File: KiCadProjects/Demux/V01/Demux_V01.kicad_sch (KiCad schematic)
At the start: 40 parts, among them J1 alimentacao analogica, J12 +9Vmux, J13 +5Vmux, J14 +3.3Vmux, J15 -9Vmux, J16 -5Vmux, J17 GNDmux, J18 Conn_01x03, J19 Conn_01x06, J2 sinais analogicos, J20 Conn_01x06, J21 Conn_01x06, J22 Conn_01x06, J23 Conn_01x06, J24 Conn_01x06, J25 Conn_01x06, J26 Conn_01x06, J27 Conn_01x06, J28 Conn_01x06, J29 Conn_01x06, J3 comunicacao / sinais digitais, J30 Conn_01x06, J31 Conn_01x06, J32 Conn_01x06, J33 Conn_01x06, J34 Conn_01x06, J4 Conn_01x02, J5 Conn_01x02, J6 Conn_01x02, U1A1 74HC4051, U1B1 74HC4051, U2 BluePill_STM32F103C, U2A2 74HC4051, U2B2 74HC4051, U3A3 74HC4051, U3B3 74HC4051, U4A4 74HC4051, U4B4 74HC4051, U5A1 74HC4051, U5B1 74HC4051

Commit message: modificar
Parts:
- J12, J13, J14, J15, J16, J17, J4, J5, J6: footprint (none) -> Connector_PinHeader_2.54mm:PinHeader_1x02_P2.54mm_Vertical
- J18: footprint (none) -> Connector_PinHeader_2.54mm:PinHeader_1x03_P2.54mm_Vertical
- J19, J20, J21, J22, J23, J24, J25, J26, J27, J28, J29, J30, J31, J32, J33, J34: footprint (none) -> Connector_PinHeader_2.54mm:PinHeader_1x06_P2.54mm_Horizontal
- U1A1, U1B1, U2A2, U2B2, U3A3, U3B3, U4A4, U4B4, U5A1, U5B1: footprint (none) -> 74HC4051N:N16
- U2: footprint BluePill_breakouts:BluePill_STM32F103C -> BluePill_STM32:BluePill_STM32F103C
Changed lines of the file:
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@@
       (effects (font (size 1.27 1.27)))
     )
-    (property "Footprint" "" (at 224.663 51.181 0)
+    (property "Footprint" "Connector_PinHeader_2.54mm:PinHeader_1x06_P2.54mm_Horizontal" (at 224.663 51.181 0)
       (effects (font (size 1.27 1.27)) hide)
     )
@@
       (effects (font (size 1.27 1.27)) (justify left))
     )
-    (property "Footprint" "" (at 26.924 60.706 0)
+    (property "Footprint" "74HC4051N:N16" (at 26.924 60.706 0)
       (effects (font (size 1.27 1.27)) hide)
     )
@@
       (effects (font (size 1.27 1.27)))
     )
-    (property "Footprint" "" (at 257.302 25.781 0)
+    (property "Footprint" "Connector_PinHeader_2.54mm:PinHeader_1x06_P2.54mm_Horizontal" (at 257.302 25.781 0)
       (effects (font (size 1.27 1.27)) hide)
     )
@@
       (effects (font (size 1.27 1.27)))
     )
-    (property "Footprint" "" (at 144.272 122.428 0)
+    (property "Footprint" "Connector_PinHeader_2.54mm:PinHeader_1x02_P2.54mm_Vertical" (at 144.272 122.428 0)
       (effects (font (size 1.27 1.27)) hide)
     )
@@
       (effects (font (size 1.27 1.27)))
     )
-    (property "Footprint" "" (at 224.663 25.654 0)
+    (property "Footprint" "Connector_PinHeader_2.54mm:PinHeader_1x06_P2.54mm_Horizontal" (at 224.663 25.654 0)
       (effects (font (size 1.27 1.27)) hide)
     )
@@
       (effects (font (size 1.27 1.27)) (justify left))
     )
-    (property "Footprint" "" (at 27.432 134.874 0)
+    (property "Footprint" "74HC4051N:N16" (at 27.432 134.874 0)
       (effects (font (size 1.27 1.27)) hide)
     )
@@
       (effects (font (size 1.27 1.27)))
     )
-    (property "Footprint" "" (at 273.685 25.781 0)
+    (property "Footprint" "Connector_PinHeader_2.54mm:PinHeader_1x06_P2.54mm_Horizontal" (at 273.685 25.781 0)
       (effects (font (size 1.27 1.27)) hide)
     )
@@
       (effects (font (size 1.27 1.27)))
     )
-    (property "Footprint" "" (at 273.685 51.308 0)
+    (property "Footprint" "Connector_PinHeader_2.54mm:PinHeader_1x06_P2.54mm_Horizontal" (at 273.685 51.308 0)
       (effects (font (size 1.27 1.27)) hide)
     )
@@
       (effects (font (size 1.27 1.27)) (justify left))
     )
-    (property "Footprint" "" (at 107.95 77.724 0)
+    (property "Footprint" "74HC4051N:N16" (at 107.95 77.724 0)
       (effects (font (size 1.27 1.27)) hide)
     )
@@
       (effects (font (size 1.27 1.27)) (justify left))
     )
-    (property "Footprint" "" (at 103.378 156.972 0)
+    (property "Footprint" "74HC4051N:N16" (at 103.378 156.972 0)
       (effects (font (size 1.27 1.27)) hide)
     )
@@
       (effects (font (size 1.27 1.27)))
     )
-    (property "Footprint" "" (at 179.324 125.984 0)
+    (property "Footprint" "Connector_PinHeader_2.54mm:PinHeader_1x02_P2.54mm_Vertical" (at 179.324 125.984 0)
       (effects (font (size 1.27 1.27)) hide)
     )
@@
       (effects (font (size 1.27 1.27)))
     )
-    (property "Footprint" "" (at 224.409 75.5142 0)
+    (property "Footprint" "Connector_PinHeader_2.54mm:PinHeader_1x06_P2.54mm_Horizontal" (at 224.409 75.5142 0)
       (effects (font (size 1.27 1.27)) hide)
     )
@@
       (effects (font (size 1.27 1.27)))
     )
-    (property "Footprint" "BluePill_breakouts:BluePill_STM32F103C" (at 164.592 16.256 0)
+    (property "Footprint" "BluePill_STM32:BluePill_STM32F103C" (at 164.592 16.256 0)
       (effects (font (size 1.27 1.27)) hide)
     )
@@
       (effects (font (size 1.27 1.27)) (justify left))
     )
-    (property "Footprint" "" (at 65.786 74.168 0)
+    (property "Footprint" "74HC4051N:N16" (at 65.786 74.168 0)
       (effects (font (size 1.27 1.27)) hide)
     )
@@
       (effects (font (size 1.27 1.27)))
     )
-    (property "Footprint" "" (at 160.528 147.574 0)
+    (property "Footprint" "Connector_PinHeader_2.54mm:PinHeader_1x02_P2.54mm_Vertical" (at 160.528 147.574 0)
       (effects (font (size 1.27 1.27)) hide)
     )
@@
       (effects (font (size 1.27 1.27)) (justify left))
     )
-    (property "Footprint" "" (at 106.426 41.656 0)
+    (property "Footprint" "74HC4051N:N16" (at 106.426 41.656 0)
       (effects (font (size 1.27 1.27)) hide)
     )
@@
       (effects (font (size 1.27 1.27)))
     )
-    (property "Footprint" "" (at 150.114 147.574 0)
+    (property "Footprint" "Connector_PinHeader_2.54mm:PinHeader_1x02_P2.54mm_Vertical" (at 150.114 147.574 0)
       (effects (font (size 1.27 1.27)) hide)
     )
@@
       (effects (font (size 1.27 1.27)) (justify left))
     )
-    (property "Footprint" "" (at 63.246 113.792 0)
+    (property "Footprint" "74HC4051N:N16" (at 63.246 113.792 0)
       (effects (font (size 1.27 1.27)) hide)
     )
@@
       (effects (font (size 1.27 1.27)))
     )
-    (property "Footprint" "" (at 155.956 122.682 0)
+    (property "Footprint" "Connector_PinHeader_2.54mm:PinHeader_1x02_P2.54mm_Vertical" (at 155.956 122.682 0)
       (effects (font (size 1.27 1.27)) hide)
     )
@@
       (effects (font (size 1.27 1.27)))
     )
-    (property "Footprint" "" (at 257.048 75.6412 0)
+    (property "Footprint" "Connector_PinHeader_2.54mm:PinHeader_1x06_P2.54mm_Horizontal" (at 257.048 75.6412 0)
       (effects (font (size 1.27 1.27)) hide)
     )
@@
       (effects (font (size 1.27 1.27)))
     )
-    (property "Footprint" "" (at 240.919 25.654 0)
+    (property "Footprint" "Connector_PinHeader_2.54mm:PinHeader_1x06_P2.54mm_Horizontal" (at 240.919 25.654 0)
       (effects (font (size 1.27 1.27)) hide)
     )
@@
       (effects (font (size 1.27 1.27)))
     )
-    (property "Footprint" "" (at 131.318 122.682 0)
+    (property "Footprint" "Connector_PinHeader_2.54mm:PinHeader_1x02_P2.54mm_Vertical" (at 131.318 122.682 0)
       (effects (font (size 1.27 1.27)) hide)
     )
@@
       (effects (font (size 1.27 1.27)) (justify left))
     )
-    (property "Footprint" "" (at 62.23 153.162 0)
+    (property "Footprint" "74HC4051N:N16" (at 62.23 153.162 0)
       (effects (font (size 1.27 1.27)) hide)
     )
@@
       (effects (font (size 1.27 1.27)))
     )
-    (property "Footprint" "" (at 171.704 148.082 0)
+    (property "Footprint" "Connector_PinHeader_2.54mm:PinHeader_1x02_P2.54mm_Vertical" (at 171.704 148.082 0)
       (effects (font (size 1.27 1.27)) hide)
     )
@@
       (effects (font (size 1.27 1.27)))
     )
-    (property "Footprint" "" (at 240.919 51.181 0)
+    (property "Footprint" "Connector_PinHeader_2.54mm:PinHeader_1x06_P2.54mm_Horizontal" (at 240.919 51.181 0)
       (effects (font (size 1.27 1.27)) hide)
     )
@@
       (effects (font (size 1.27 1.27)))
     )
-    (property "Footprint" "" (at 224.536 97.79 0)
+    (property "Footprint" "Connector_PinHeader_2.54mm:PinHeader_1x06_P2.54mm_Horizontal" (at 224.536 97.79 0)
       (effects (font (size 1.27 1.27)) hide)
     )
@@
       (effects (font (size 1.27 1.27)))
     )
-    (property "Footprint" "" (at 166.37 126.238 0)
+    (property "Footprint" "Connector_PinHeader_2.54mm:PinHeader_1x02_P2.54mm_Vertical" (at 166.37 126.238 0)
       (effects (font (size 1.27 1.27)) hide)
     )
@@
       (effects (font (size 1.27 1.27)))
     )
-    (property "Footprint" "" (at 273.812 98.044 0)
+    (property "Footprint" "Connector_PinHeader_2.54mm:PinHeader_1x06_P2.54mm_Horizontal" (at 273.812 98.044 0)
       (effects (font (size 1.27 1.27)) hide)
     )
@@
       (effects (font (size 1.27 1.27)) (justify left))
     )
-    (property "Footprint" "" (at 30.988 106.172 0)
+    (property "Footprint" "Connector_PinHeader_2.54mm:PinHeader_1x03_P2.54mm_Vertical" (at 30.988 106.172 0)
       (effects (font (size 1.27 1.27)) hide)
     )
@@
       (effects (font (size 1.27 1.27)))
     )
-    (property "Footprint" "" (at 240.3856 75.4888 0)
+    (property "Footprint" "Connector_PinHeader_2.54mm:PinHeader_1x06_P2.54mm_Horizontal" (at 240.3856 75.4888 0)
       (effects (font (size 1.27 1.27)) hide)
     )
@@
       (effects (font (size 1.27 1.27)))
     )
-    (property "Footprint" "" (at 273.05 75.692 0)
+    (property "Footprint" "Connector_PinHeader_2.54mm:PinHeader_1x06_P2.54mm_Horizontal" (at 273.05 75.692 0)
       (effects (font (size 1.27 1.27)) hide)
     )
@@
       (effects (font (size 1.27 1.27)))
     )
-    (property "Footprint" "" (at 257.302 51.308 0)
+    (property "Footprint" "Connector_PinHeader_2.54mm:PinHeader_1x06_P2.54mm_Horizontal" (at 257.302 51.308 0)
       (effects (font (size 1.27 1.27)) hide)
     )
@@
       (effects (font (size 1.27 1.27)))
     )
-    (property "Footprint" "" (at 257.302 97.79 0)
+    (property "Footprint" "Connector_PinHeader_2.54mm:PinHeader_1x06_P2.54mm_Horizontal" (at 257.302 97.79 0)
       (effects (font (size 1.27 1.27)) hide)
     )
@@
       (effects (font (size 1.27 1.27)) (justify left))
     )
-    (property "Footprint" "" (at 102.108 118.872 0)
+    (property "Footprint" "74HC4051N:N16" (at 102.108 118.872 0)
       (effects (font (size 1.27 1.27)) hide)
     )
@@
       (effects (font (size 1.27 1.27)))
     )
-    (property "Footprint" "" (at 240.792 97.79 0)
+    (property "Footprint" "Connector_PinHeader_2.54mm:PinHeader_1x06_P2.54mm_Horizontal" (at 240.792 97.79 0)
       (effects (font (size 1.27 1.27)) hide)
     )
@@
       (effects (font (size 1.27 1.27)) (justify left))
     )
-    (property "Footprint" "" (at 66.04 39.624 0)
+    (property "Footprint" "74HC4051N:N16" (at 66.04 39.624 0)
       (effects (font (size 1.27 1.27)) hide)
     )
@@
       (effects (font (size 1.27 1.27)))
     )
-    (property "Footprint" "" (at 191.008 126.238 0)
+    (property "Footprint" "Connector_PinHeader_2.54mm:PinHeader_1x02_P2.54mm_Vertical" (at 191.008 126.238 0)
       (effects (font (size 1.27 1.27)) hide)
     )

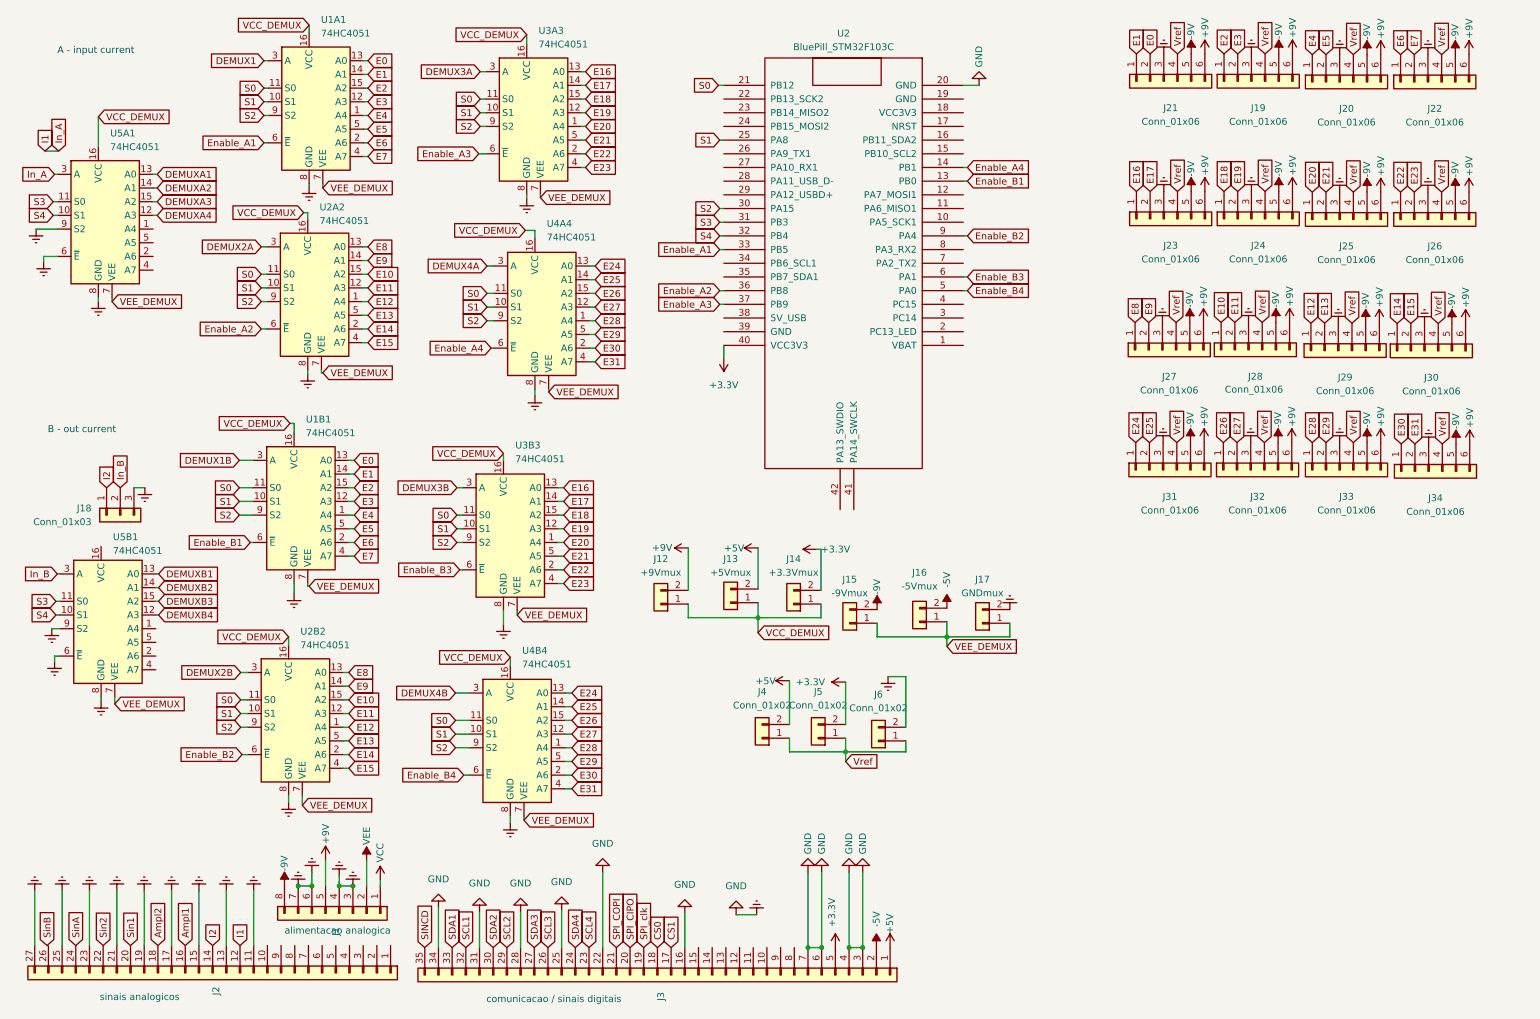
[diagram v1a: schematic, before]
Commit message: placa em producao
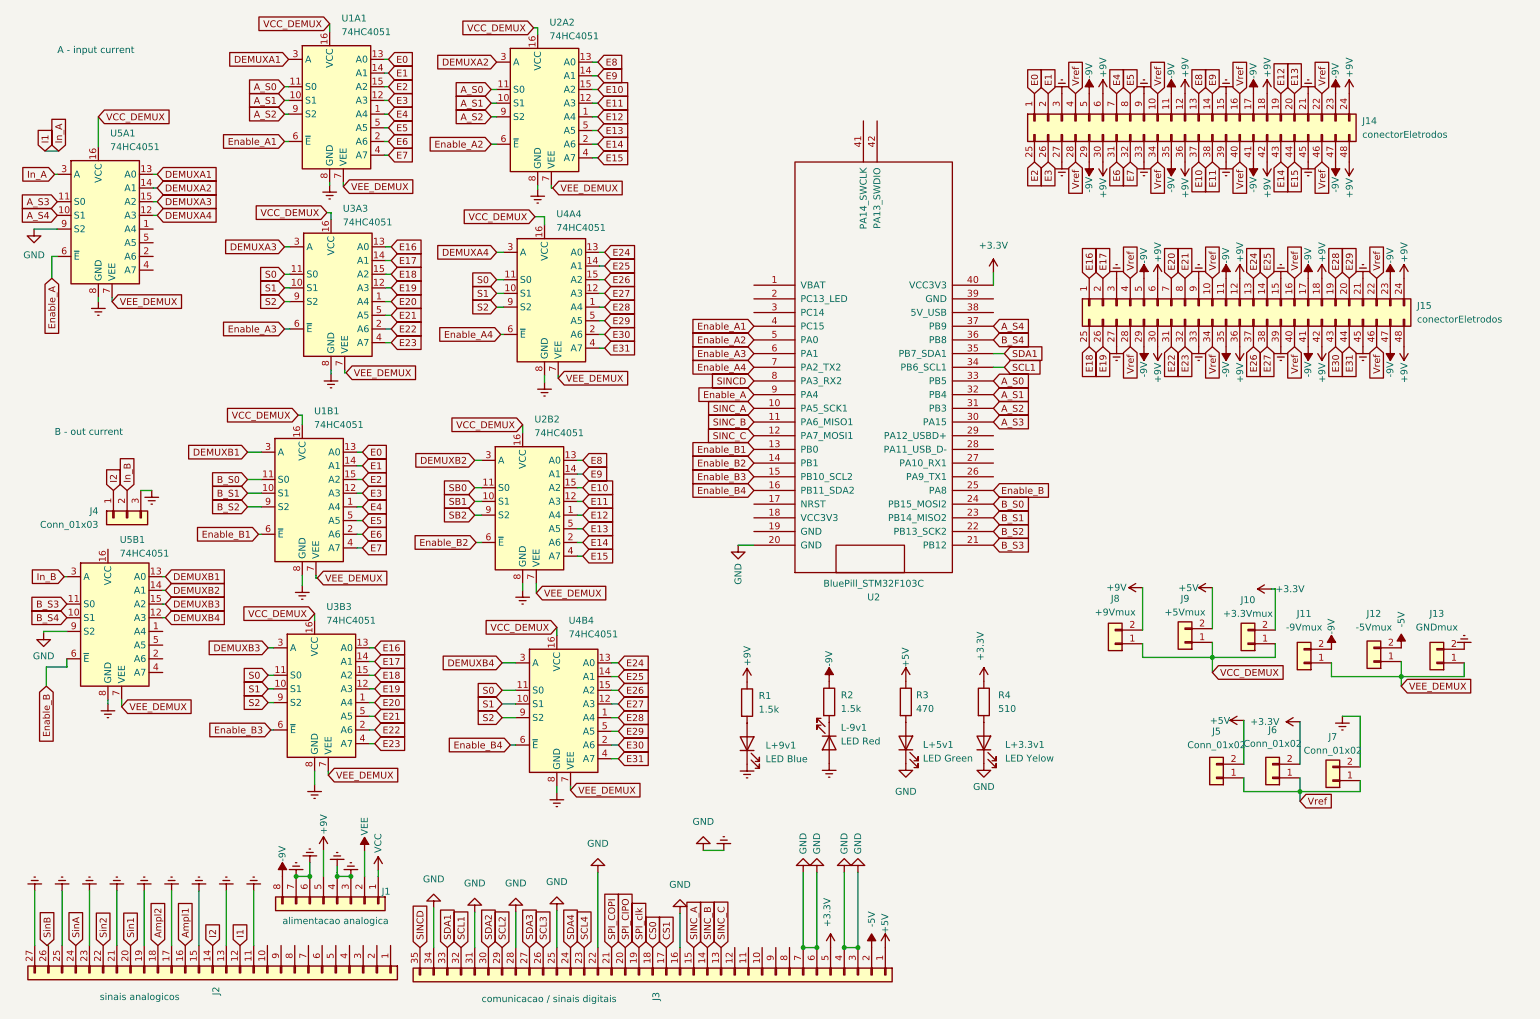
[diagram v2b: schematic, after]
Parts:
- removed J19, J20, J21, J22, J23, J24, J25, J26, J27, J28, J29, J30, J31, J32, J33, J34: Conn_01x06, Connector_PinHeader_2.54mm:PinHeader_1x06_P2.54mm_Horizontal, symbol Connector_Generic:Conn_01x06
- added J14, J15: conectorEletrodos, Connector_PinHeader_2.54mm:PinHeader_2x24_P2.54mm_Vertical, symbol Connector_Generic:Conn_02x24_Top_Bottom
- added L+3.3v1: LED Yelow, LED_THT:LED_D5.0mm, symbol Device:LED
- added L+5v1: LED Green, LED_THT:LED_D5.0mm, symbol Device:LED
- added L+9v1: LED Blue, LED_THT:LED_D5.0mm, symbol Device:LED
- added L-9v1: LED Red, LED_THT:LED_D5.0mm, symbol Device:LED
- added R1, R2: 1.5k, Resistor_THT:R_Axial_DIN0207_L6.3mm_D2.5mm_P7.62mm_Horizontal, symbol Device:R
- added R3: 470, Resistor_THT:R_Axial_DIN0207_L6.3mm_D2.5mm_P7.62mm_Horizontal, symbol Device:R
- added R4: 510, Resistor_THT:R_Axial_DIN0207_L6.3mm_D2.5mm_P7.62mm_Horizontal, symbol Device:R
- renumbered J14 to J10, J15 to J11, J16 to J12, J17 to J13, J18 to J4, J4 to J5, J5 to J6, J6 to J7, J12 to J8, J13 to J9
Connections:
- net DEMUX1 is gone; now on net DEMUXA1: U1A1.3 (A)
- net DEMUX1B is gone; now on net DEMUXB1: U1B1.3 (A)
- net DEMUX2A is gone; now on net DEMUXA2: U2A2.3 (A)
- net DEMUX2B is gone; now on net DEMUXB2: U2B2.3 (A)
- net DEMUX3A is gone; now on net DEMUXA3: U3A3.3 (A)
- net DEMUX3B is gone; now on net DEMUXB3: U3B3.3 (A)
- net DEMUX4A is gone; now on net DEMUXA4: U4A4.3 (A)
- net DEMUX4B is gone; now on net DEMUXB4: U4B4.3 (A)
- net +3.3V: now also R4.1
- net +5V: now also R3.1
- net +9V: now also J14.12 (Pin_12), J14.18 (Pin_18), J14.24 (Pin_24), J14.30 (Pin_30), J14.36 (Pin_36), J14.42 (Pin_42), J14.48 (Pin_48), J14.6 (Pin_6), J15.12 (Pin_12), J15.18 (Pin_18), J15.24 (Pin_24), J15.30 (Pin_30), J15.36 (Pin_36), J15.42 (Pin_42), J15.48 (Pin_48), J15.6 (Pin_6), R1.1
- net -9V: now also J14.11 (Pin_11), J14.17 (Pin_17), J14.23 (Pin_23), J14.29 (Pin_29), J14.35 (Pin_35), J14.41 (Pin_41), J14.47 (Pin_47), J14.5 (Pin_5), J15.11 (Pin_11), J15.17 (Pin_17), J15.23 (Pin_23), J15.29 (Pin_29), J15.35 (Pin_35), J15.41 (Pin_41), J15.47 (Pin_47), J15.5 (Pin_5), R2.1
- net E0: now also J14.1 (Pin_1)
- net E1: now also J14.2 (Pin_2)
- net E10: now also J14.37 (Pin_37)
- net E11: now also J14.38 (Pin_38)
- net E12: now also J14.19 (Pin_19)
- net E13: now also J14.20 (Pin_20)
- net E14: now also J14.43 (Pin_43)
- net E15: now also J14.44 (Pin_44)
- net E16: now also J15.1 (Pin_1)
- net E17: now also J15.2 (Pin_2)
- net E18: now also J15.25 (Pin_25)
- net E19: now also J15.26 (Pin_26)
- net E2: now also J14.25 (Pin_25)
- net E20: now also J15.7 (Pin_7)
- net E21: now also J15.8 (Pin_8)
- net E22: now also J15.31 (Pin_31)
- net E23: now also J15.32 (Pin_32)
- net E24: now also J15.13 (Pin_13)
- net E25: now also J15.14 (Pin_14)
- net E26: now also J15.37 (Pin_37)
- net E27: now also J15.38 (Pin_38)
- net E28: now also J15.19 (Pin_19)
- net E29: now also J15.20 (Pin_20)
- net E3: now also J14.26 (Pin_26)
- net E30: now also J15.43 (Pin_43)
- net E31: now also J15.44 (Pin_44)
- net E4: now also J14.7 (Pin_7)
- net E5: now also J14.8 (Pin_8)
- net E6: now also J14.31 (Pin_31)
- net E7: now also J14.32 (Pin_32)
- net E8: now also J14.13 (Pin_13)
- net E9: now also J14.14 (Pin_14)
- net Earth: now also J14.15 (Pin_15), J14.21 (Pin_21), J14.27 (Pin_27), J14.3 (Pin_3), J14.33 (Pin_33), J14.39 (Pin_39), J14.45 (Pin_45), J14.9 (Pin_9), J15.15 (Pin_15), J15.21 (Pin_21), J15.27 (Pin_27), J15.3 (Pin_3), J15.33 (Pin_33), J15.39 (Pin_39), J15.45 (Pin_45), J15.9 (Pin_9), L+3.3v1.1 (K), L+5v1.1 (K), L+9v1.1 (K), L-9v1.2 (A); no longer U5A1.6 (~{E}), U5B1.6 (~{E})
- net Enable_A1: now also U2.4 (PC15); no longer U2.33 (PB5)
- net Enable_A2: now also U2.5 (PA0); no longer U2.36 (PB8)
- net Enable_A3: now also U2.6 (PA1); no longer U2.37 (PB9)
- net Enable_A4: now also U2.7 (PA2_TX2); no longer U2.14 (PB1)
- net Enable_B2: now also U2.14 (PB1); no longer U2.9 (PA4)
- net Enable_B3: now also U2.15 (PB10_SCL2); no longer U2.6 (PA1)
- net Enable_B4: now also U2.16 (PB11_SDA2); no longer U2.5 (PA0)
- net S0: no longer U1A1.11 (S0), U1B1.11 (S0), U2.21 (PB12), U2A2.11 (S0), U2B2.11 (S0)
- net S1: no longer U1A1.10 (S1), U1B1.10 (S1), U2.25 (PA8), U2A2.10 (S1), U2B2.10 (S1)
- net S2: no longer U1A1.9 (S2), U1B1.9 (S2), U2.30 (PA15), U2A2.9 (S2), U2B2.9 (S2)
- net SCL1: now also U2.34 (PB6_SCL1)
- net SDA1: now also U2.35 (PB7_SDA1)
- net SINCD: now also U2.8 (PA3_RX2)
- net Vref: now also J14.10 (Pin_10), J14.16 (Pin_16), J14.22 (Pin_22), J14.28 (Pin_28), J14.34 (Pin_34), J14.4 (Pin_4), J14.40 (Pin_40), J14.46 (Pin_46), J15.10 (Pin_10), J15.16 (Pin_16), J15.22 (Pin_22), J15.28 (Pin_28), J15.34 (Pin_34), J15.4 (Pin_4), J15.40 (Pin_40), J15.46 (Pin_46)
- net SINC_A: now reaches U2.10 (PA5_SCK1)
- net SINC_A: now also J3.15 (Pin_15)
- net SINC_B: now reaches U2.11 (PA6_MISO1)
- net SINC_B: now also J3.14 (Pin_14)
- net SINC_C: now reaches U2.12 (PA7_MOSI1)
- net SINC_C: now also J3.13 (Pin_13)
- net B_S2: now reaches U2.22 (PB13_SCK2)
- net B_S2: now also U1B1.9 (S2)
- net B_S1: now reaches U2.23 (PB14_MISO2)
- net B_S1: now also U1B1.10 (S1)
- net B_S0: now reaches U2.24 (PB15_MOSI2)
- net B_S0: now also U1B1.11 (S0)
- removed net S3: U2.31 (PB3), U5A1.11 (S0), U5B1.11 (S0)
- removed net S4: U2.32 (PB4), U5A1.10 (S1), U5B1.10 (S1)
- new net: L-9v1.1 (K), R2.2
- new net: L+3.3v1.2 (A), R4.2
- new net: L+9v1.2 (A), R1.2
- new net: L+5v1.2 (A), R3.2
- new net A_S0: U1A1.11 (S0), U2.33 (PB5), U2A2.11 (S0)
- new net A_S1: U1A1.10 (S1), U2.32 (PB4), U2A2.10 (S1)
- new net A_S2: U1A1.9 (S2), U2.31 (PB3), U2A2.9 (S2)
- new net A_S3: U2.30 (PA15), U5A1.11 (S0)
- new net A_S4: U2.37 (PB9), U5A1.10 (S1)
- new net B_S3: U2.21 (PB12), U5B1.11 (S0)
- new net B_S4: U2.36 (PB8), U5B1.10 (S1)
- new net Enable_A: U2.9 (PA4), U5A1.6 (~{E})
- new net Enable_B: U2.25 (PA8), U5B1.6 (~{E})
- new net SB0: U2B2.11 (S0)
- new net SB1: U2B2.10 (S1)
- new net SB2: U2B2.9 (S2)
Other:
- company: EITduino -> Autor: Gustavo Pinheiro
- title: Barramento V04 -> Demux
- moved on the sheet: J1, J10, J11, J12, J13, J3, J4, J5, J6, J7, J8, J9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
